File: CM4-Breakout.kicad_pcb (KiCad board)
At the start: 2 copper layers, 17 parts, among them J1 Conn_01x10_Male, J10 Conn_01x12_Male, J11 Conn_01x12_Male, J12 Conn_01x08_Male, J13 Conn_01x03_Male, J14 Conn_01x02_Female, J15 Conn_01x04_Male, J2 Conn_01x13_Male, J3 Conn_01x12_Male, J4 Conn_01x13_Male, J5 Conn_01x13_Male, J6 Conn_01x04_Male, J7 Conn_01x03_Male, J8 Conn_01x17_Male, J9 Conn_01x16_Male

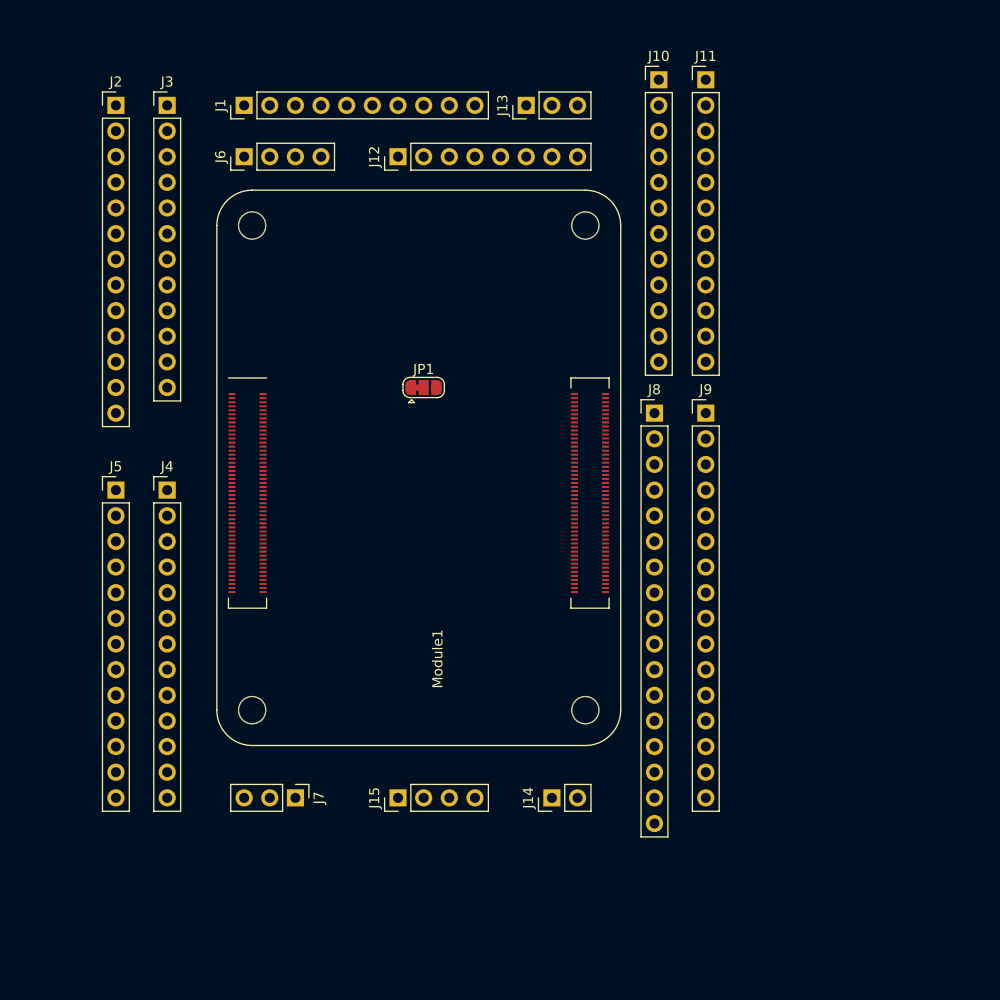
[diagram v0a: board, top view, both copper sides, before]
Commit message: Final
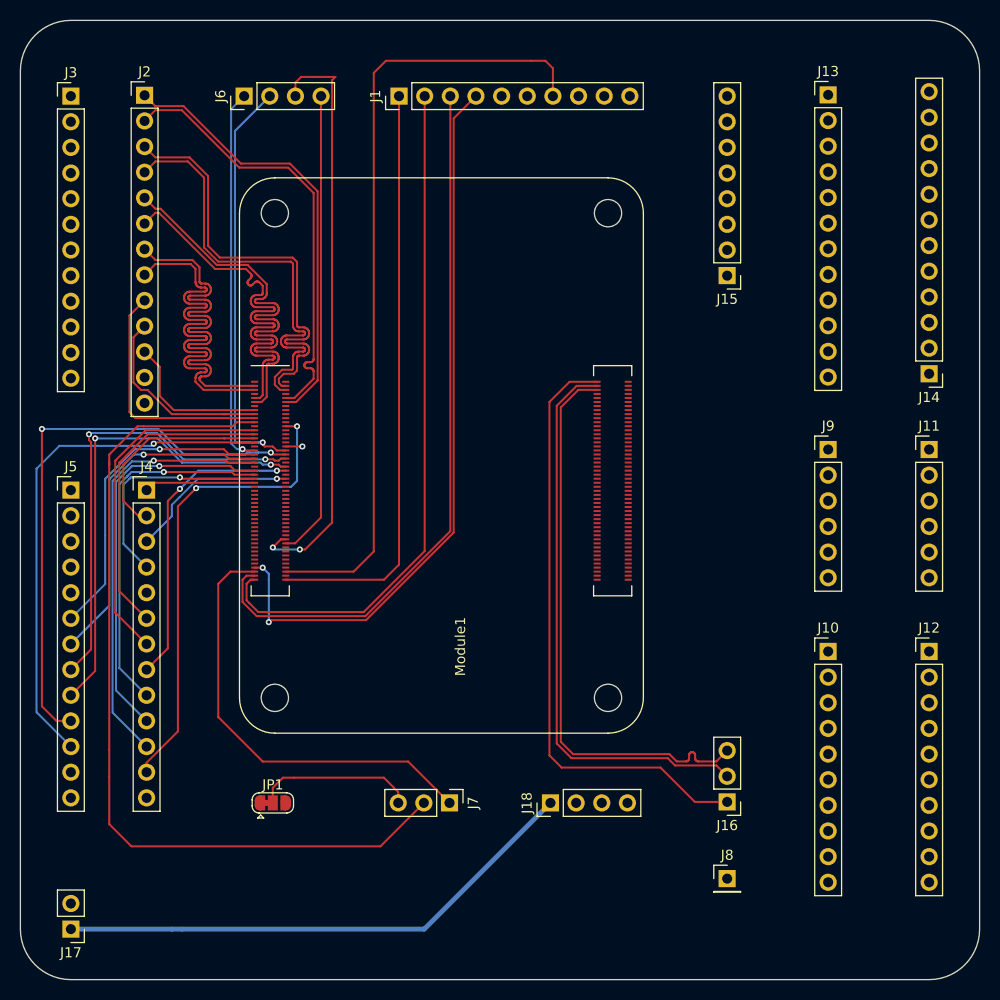
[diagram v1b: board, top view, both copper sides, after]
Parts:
- added J16: Conn_01x03_Male, Connector_PinHeader_2.54mm:PinHeader_1x03_P2.54mm_Vertical, F.Cu at (185.0, 127.4)
- added J17: Conn_01x02_Female, Connector_PinHeader_2.54mm:PinHeader_1x02_P2.54mm_Vertical, F.Cu at (120.0, 140.0)
- added J18: Conn_01x04_Male, Connector_PinHeader_2.54mm:PinHeader_1x04_P2.54mm_Vertical, F.Cu at (167.5, 127.5)
- J10: value Conn_01x12_Male -> Conn_01x10_Male; footprint Connector_PinHeader_2.54mm:PinHeader_1x12_P2.54mm_Vertical -> Connector_PinHeader_2.54mm:PinHeader_1x10_P2.54mm_Vertical
- J11: value Conn_01x12_Male -> Conn_01x06_Male; footprint Connector_PinHeader_2.54mm:PinHeader_1x12_P2.54mm_Vertical -> Connector_PinHeader_2.54mm:PinHeader_1x06_P2.54mm_Vertical
- J12: value Conn_01x08_Male -> Conn_01x10_Male; footprint Connector_PinHeader_2.54mm:PinHeader_1x08_P2.54mm_Vertical -> Connector_PinHeader_2.54mm:PinHeader_1x10_P2.54mm_Vertical
- J13: value Conn_01x03_Male -> Conn_01x12_Male; footprint Connector_PinHeader_2.54mm:PinHeader_1x03_P2.54mm_Vertical -> Connector_PinHeader_2.54mm:PinHeader_1x12_P2.54mm_Vertical
- J14: value Conn_01x02_Female -> Conn_01x12_Male; footprint Connector_PinHeader_2.54mm:PinHeader_1x02_P2.54mm_Vertical -> Connector_PinHeader_2.54mm:PinHeader_1x12_P2.54mm_Vertical
- J15: value Conn_01x04_Male -> Conn_01x08_Male; footprint Connector_PinHeader_2.54mm:PinHeader_1x04_P2.54mm_Vertical -> Connector_PinHeader_2.54mm:PinHeader_1x08_P2.54mm_Vertical
- J8: value Conn_01x17_Male -> Conn_01x01_Male; footprint Connector_PinHeader_2.54mm:PinHeader_1x17_P2.54mm_Vertical -> Connector_PinHeader_2.54mm:PinHeader_1x01_P2.54mm_Vertical
- J9: value Conn_01x16_Male -> Conn_01x06_Male; footprint Connector_PinHeader_2.54mm:PinHeader_1x16_P2.54mm_Vertical -> Connector_PinHeader_2.54mm:PinHeader_1x06_P2.54mm_Vertical
- moved J12 71.9 mm to (205.0, 112.5), turned to 0 degrees
- moved J15 61.1 mm to (185.0, 75.3), turned to 180 degrees
- moved J10 59.1 mm to (195.0, 112.5)
- moved J14 56.2 mm to (205.0, 85.0), turned to 180 degrees
- moved J8 46.7 mm to (185.0, 135.0)
- moved JP1 43.8 mm to (140.0, 127.5)
- moved J11 42.8 mm to (205.0, 92.5)
- moved J13 29.9 mm to (195.0, 57.4), turned to 0 degrees
- moved J1 15.4 mm to (152.5, 57.5)
- moved J7 15.3 mm to (157.5, 127.5)
- moved J9 12.6 mm to (195.0, 92.5)
- moved J3 9.58 mm to (120.0, 57.5)
- moved J6 6.00 mm to (137.2, 57.5)
- moved J5 4.46 mm to (120.0, 96.5)
- moved J2 3.01 mm to (127.3, 57.4)
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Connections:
- net Net-(Module1-Pad104) renamed no_connect_141
- net Net-(Module1-Pad106) renamed no_connect_142
- net Net-(Module1-Pad76) renamed no_connect_143
- J10 pad 1: /HDMI0_CEC -> /CAM1_C_N
- J10 pad 10: /HDMI0_TX1_P -> /CAM1_D3_P
- J10 pad 2: /HDMI0_CLK_N -> /CAM1_C_P
- J10 pad 3: /HDMI0_CLK_P -> /CAM1_D0_N
- J10 pad 4: /HDMI0_HOTPLUG -> /CAM1_D0_P
- J10 pad 5: /HDMI0_SCL -> /CAM1_D1_N
- J10 pad 6: /HDMI0_SDA -> /CAM1_D1_P
- J10 pad 7: /HDMI0_TX0_N -> /CAM1_D2_N
- J10 pad 8: /HDMI0_TX0_P -> /CAM1_D2_P
- J10 pad 9: /HDMI0_TX1_N -> /CAM1_D3_N
- J11 pad 1: /HDMI1_CEC -> /DSI0_C_N
- J11 pad 2: /HDMI1_CLK_N -> /DSI0_C_P
- J11 pad 3: /HDMI1_CLK_P -> /DSI0_D0_N
- J11 pad 4: /HDMI1_HOTPLUG -> /DSI0_D0_P
- J11 pad 5: /HDMI1_SCL -> /DSI0_D1_N
- J11 pad 6: /HDMI1_SDA -> /DSI0_D1_P
- J12 pad 1: /PCIe_CLK_nREQ -> /DSI1_C_N
- J12 pad 2: /PCIe_CLK_N -> /DSI1_C_P
- J12 pad 3: /PCIe_CLK_P -> /DSI1_D0_N
- J12 pad 4: /PCIe_nRST -> /DSI1_D0_P
- J12 pad 5: /PCIe_RX_N -> /DSI1_D1_N
- J12 pad 6: /PCIe_RX_P -> /DSI1_D1_P
- J12 pad 7: /PCIe_TX_N -> /DSI1_D2_N
- J12 pad 8: /PCIe_TX_P -> /DSI1_D2_P
- J13 pad 1: /USB_OTG_ID -> /HDMI0_CEC
- J13 pad 2: /USB2_N -> /HDMI0_CLK_N
- J13 pad 3: /USB2_P -> /HDMI0_CLK_P
- J14 pad 1: /+5v -> /HDMI1_CEC
- J14 pad 2: /GND -> /HDMI1_CLK_N
- J15 pad 1: /+5v -> /PCIe_CLK_nREQ
- J15 pad 2: /+3.3v -> /PCIe_CLK_N
- J15 pad 3: /+1.8v -> /PCIe_CLK_P
- J15 pad 4: /GND -> /PCIe_nRST
- J8 pad 1: /DSI0_C_N -> /VDAC_COMP
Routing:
- net /Pi_nLED_Activity: track 0.00 -> 86.4 mm
- net /AnalogIP1: track 0.00 -> 78.2 mm
- net /nRPIBOOT: track 0.00 -> 72.6 mm, vias 0 -> 2
- net /Camera_GPIO: track 0.00 -> 71.3 mm
- net /Global_EN: track 0.00 -> 68.5 mm
- net /USB_OTG_ID: track 0.00 -> 60.1 mm
- net /SCL0: track 0.00 -> 58.5 mm, vias 0 -> 2
- net /nEXTRST: track 0.00 -> 58.2 mm
- net /USB2_P: track 0.00 -> 56.5 mm
- net /USB2_N: track 0.00 -> 56.5 mm
- net /GPIO11: track 0.00 -> 56.3 mm, vias 0 -> 2
- net /+5v: track 0.00 -> 52.7 mm
- net /GPIO12: track 0.00 -> 51.6 mm, vias 0 -> 1
- net /GPIO26: track 0.00 -> 47.0 mm, vias 0 -> 2
- net /GPIO10: track 0.00 -> 46.5 mm, vias 0 -> 2
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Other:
- board outline added: 95 x 95 mm
